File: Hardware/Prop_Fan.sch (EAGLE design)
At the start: 145 parts, among them J1 1546215-2, J2 1546215-2, J3 1546215-2, J4 1546215-2, SW1 MF-SW-TACT-4.2MM, SW2 MF-SW-TACT-4.2MM, SW3 MF-SW-TACT-4.2MM, U1 P8X32A-Q44, U10 MAX31855KASA+, U11 MAX31855KASA+, U12 G3VM-61GR2(TR05), U13 G3VM-61GR2(TR05), U14 CD74HC595M96, U15 G3VM-61GR2(TR05), U16 CD74HC165M96, U17 G3VM-61GR2(TR05), U18 G3VM-61GR2(TR05), U19 G3VM-61GR2(TR05), U2 G3VM-61GR2(TR05), U20 G3VM-61GR2(TR05), U21 G3VM-61GR2(TR05), U22 G3VM-61GR2(TR05), U23 G3VM-61GR2(TR05), U24 G3VM-61GR2(TR05), U25 G3VM-61GR2(TR05), U26 G3VM-61GR2(TR05), U27 FXOS8700CQR1, U3 G3VM-61GR2(TR05), U4 MAX31855KASA+, U5 LM22678TJ-5.0/NOPB, U6 ADP3338AKCZ-3.3-RL, U7 CAT24C512WI-GT3, U8 G3VM-61GR2(TR05), U9 MAX31855KASA+, X1 ABMM-6.000MHZ-B2-T

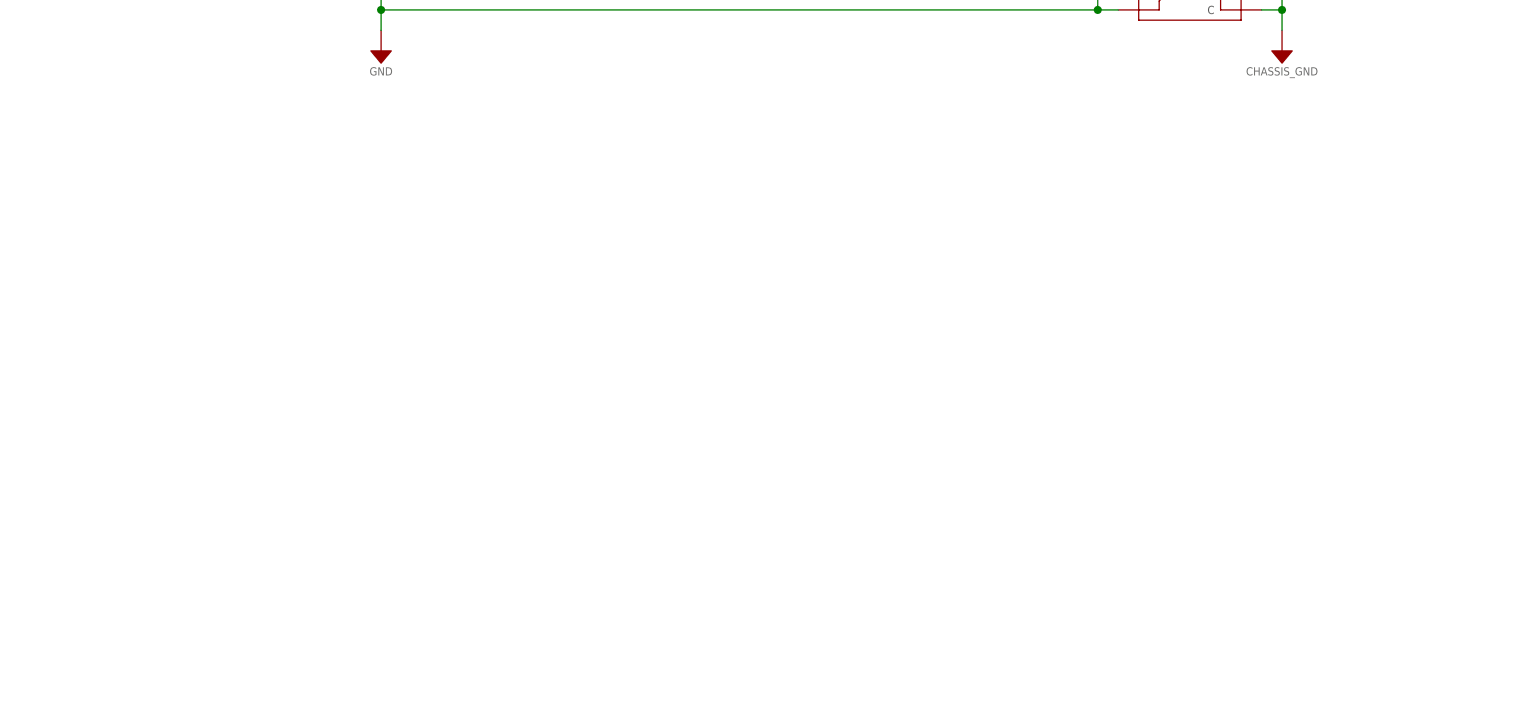
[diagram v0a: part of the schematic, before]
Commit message: PROP  Fan Rev 1 complete.
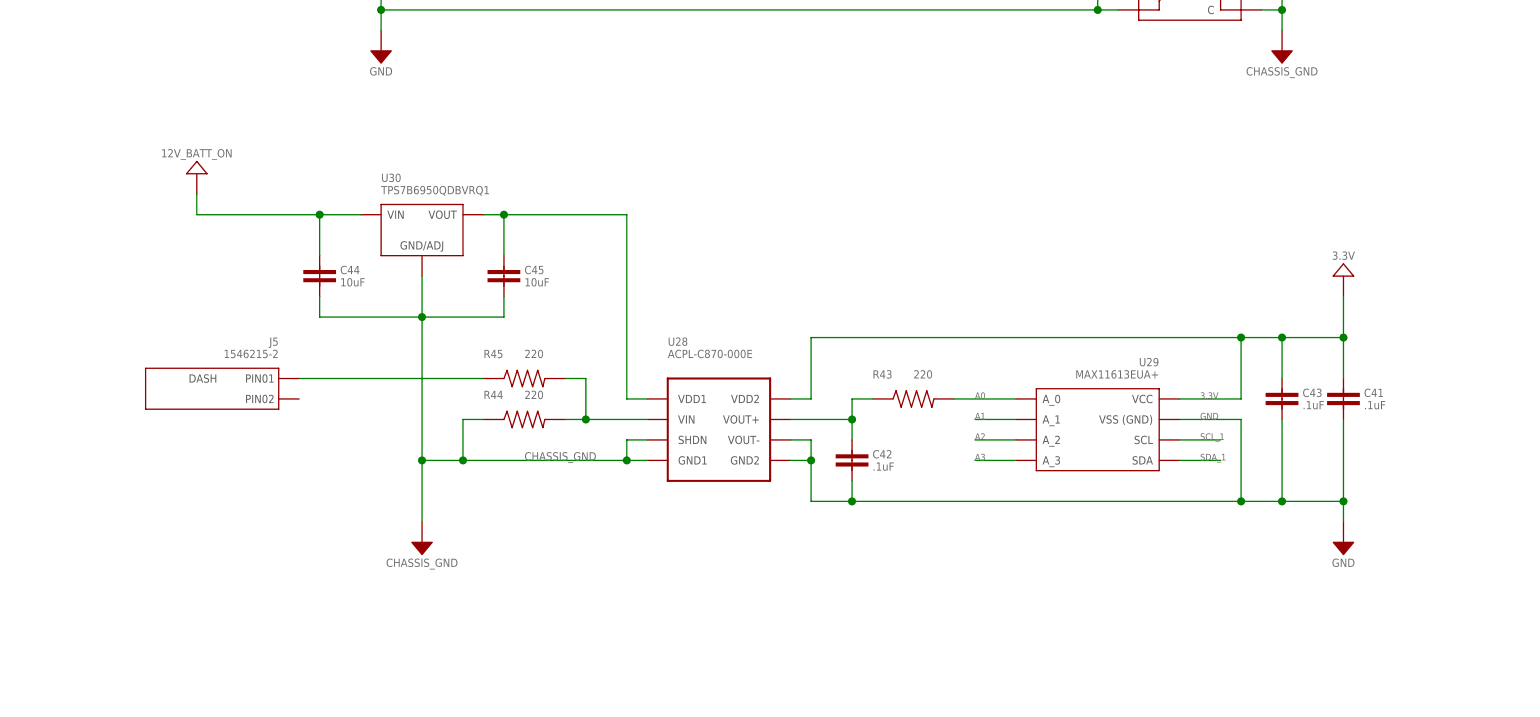
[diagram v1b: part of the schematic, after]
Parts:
- added C41, C42, C43: .1uF, PP_Passives:CAPACITOR_NON_POLAR_0603
- added C44, C45: 10uF, PP_Passives:CAPACITOR_NON_POLAR_1210
- added J5: 1546215-2, PP_Connectors:CON_01X02_1546215-2
- added R43, R44, R45: 220, MF_Passives:RESISTOR_0603
- added U28: ACPL-C870-000E, PP_AnalogIC:ACPL-C87X
- added U29: MAX11613EUA+, PP_AnalogIC:MAX11613EUA+
- added U30: TPS7B6950QDBVRQ1, MF_IC_Power:TPS7B69
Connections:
- new net A0: R43.P$2, U29.A_0
- new net A1: U29.A_1
- new net A2: U29.A_2
- new net A3: U29.A_3
- new net EXT_5V: C45.1, U28.VDD1, U30.VOUT
- new net N$32: C42.1, R43.P$1, U28.VOUT+
- new net N$33: R44.P$2, R45.P$2, U28.VIN
- new net N$36: J5.PIN1, R45.P$1
- net 12V_BATT_ON: now also C44.1, U30.VIN
- net 3.3V: now also C41.1, C43.1, U28.VDD2, U29.VCC
- net CHASSIS_GND: now also C44.2, C45.2, R44.P$1, U28.GND1, U28.SHDN, U30.GND/ADJ
- net GND: now also C41.2, C42.2, C43.2, U28.GND2, U28.VOUT-, U29.GND
- net SCL_1: now also U29.SCL
- net SDA_1: now also U29.SDA
